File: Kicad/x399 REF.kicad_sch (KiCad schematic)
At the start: 57 parts, among them J1 +15V, J2 10Vref, Q1 MMBT3904, Q2 2SD882, U1 LM399, U2 OP07

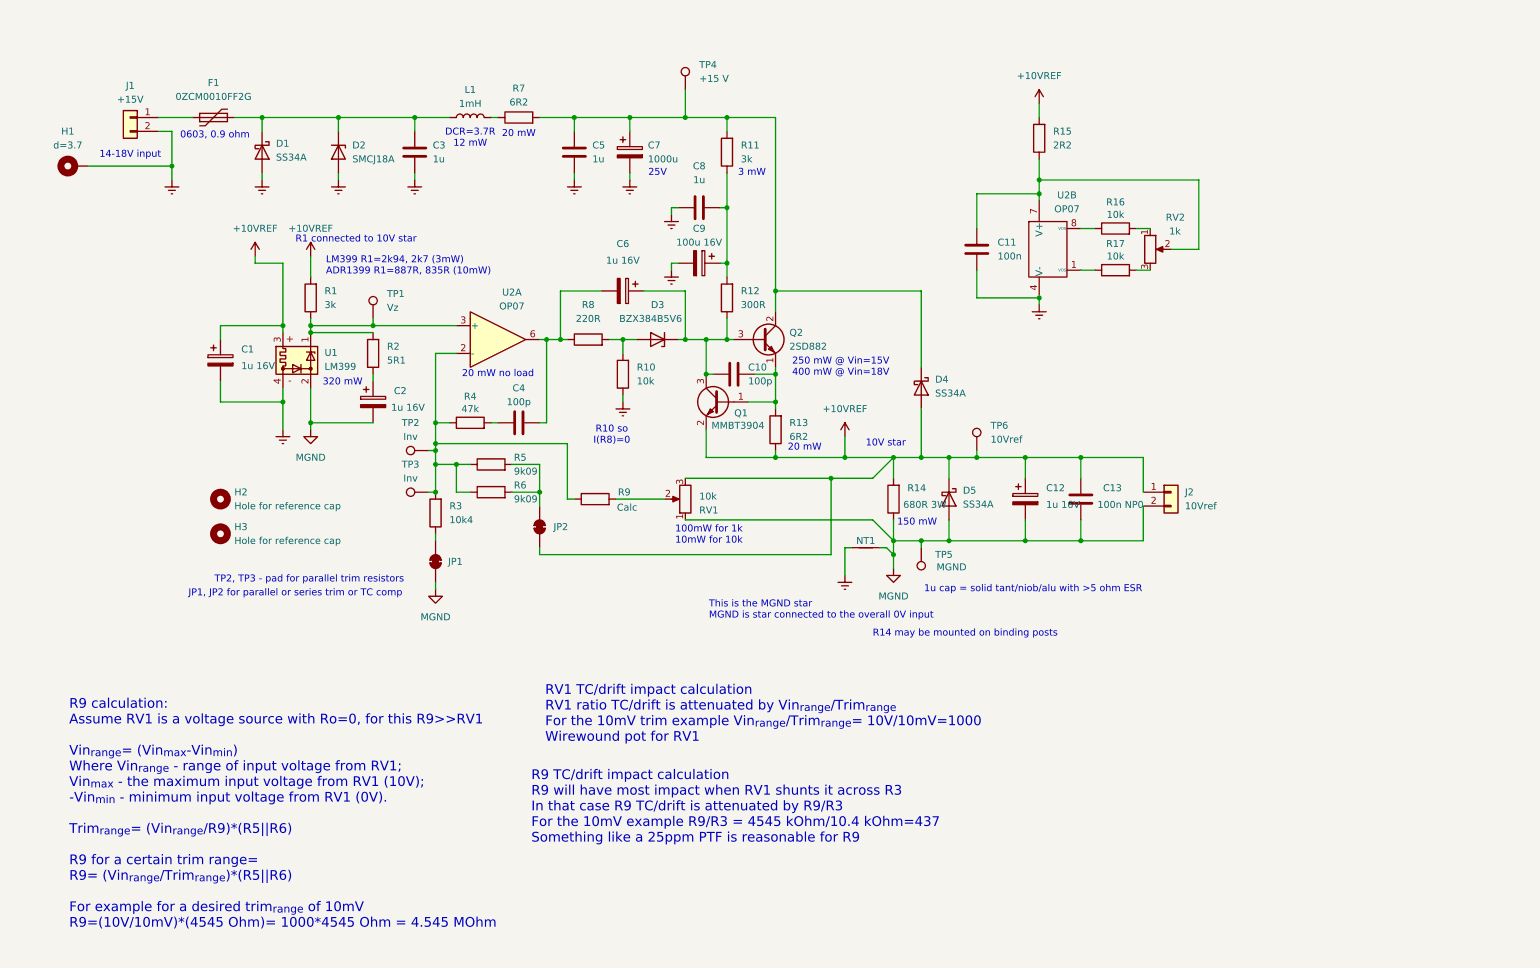
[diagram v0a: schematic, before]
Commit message: Add files via upload
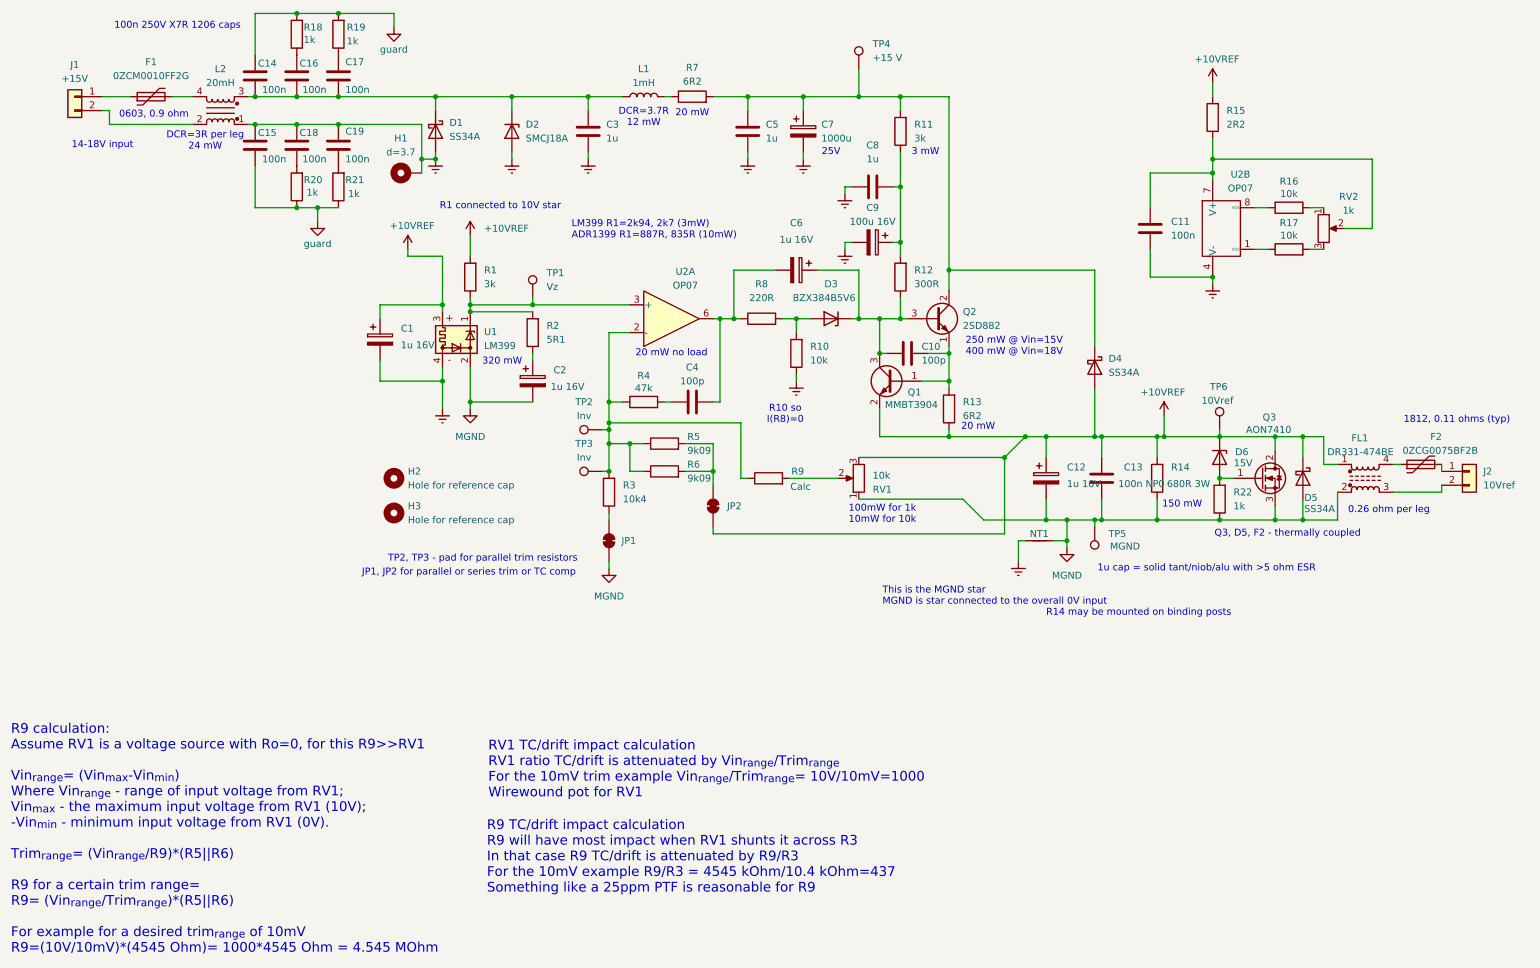
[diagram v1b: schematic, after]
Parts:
- added C14, C15, C16, C17, C18, C19: 100n, Capacitor_SMD:C_0805_2012Metric_Pad1.18x1.45mm_HandSolder, symbol Device:C
- added D6: 15V, Diode_SMD:D_SOD-323_HandSoldering, symbol Diode:BZX384xxxx
- added F2: 0ZCG0075BF2B, Resistor_SMD:R_0603_1608Metric_Pad0.98x0.95mm_HandSolder, symbol Device:Polyfuse
- added FL1: DR331-474BE, symbol Filter:Choke_CommonMode_FerriteCore_1423
- added L2: 20mH, symbol Device:Filter_EMI_CommonMode
- added Q3: AON7410, symbol Transistor_FET:Q_NMOS_GDS
- added R18, R19, R20, R21, R22: 1k, Resistor_SMD:R_0805_2012Metric_Pad1.20x1.40mm_HandSolder, symbol Device:R
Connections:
- net +10VREF: now also D6.1 (K), FL1.1, Q3.2 (D); no longer J2.1 (Pin_1)
- net Earth: now also C15.1, C18.1, C19.1, L2.1; no longer J1.2 (Pin_2)
- net MGND: now also FL1.2, Q3.3 (S), R22.1; no longer J2.2 (Pin_2)
- net at C3.1, D1.1 (K), D2.1 (K)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: now also C14.2, C16.2, C17.2, L2.3; no longer F1.2
- new net: C18.2, R20.2
- new net: C16.1, R18.1
- new net: C19.2, R21.2
- new net: D6.2 (A), Q3.1 (G), R22.2
- new net: F2.2, J2.1 (Pin_1)
- new net: FL1.3, J2.2 (Pin_2)
- new net: C17.1, R19.1
- new net: F1.2, L2.4
- new net: F2.1, FL1.4
- new net: J1.2 (Pin_2), L2.2
- new net guard: C14.1, C15.2, R18.2, R19.2, R20.1, R21.1
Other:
- note added: "0.26 ohm per leg"
- note added: "100n 250V X7R 1206 caps"
- note added: "1812, 0.11 ohms (typ)"
- note added: "DCR=3R per leg 24 mW"
- note added: "Q3, D5, F2 - thermally coupled"
- note removed: "10V star"
- moved on the sheet: C1, C10, C11, C12, C13, C2, C3, C4, C5, C6, C7, C8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
